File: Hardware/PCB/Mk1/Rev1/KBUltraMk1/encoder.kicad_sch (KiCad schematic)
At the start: 1 part, among them SW101 RotaryEncoder_Switch

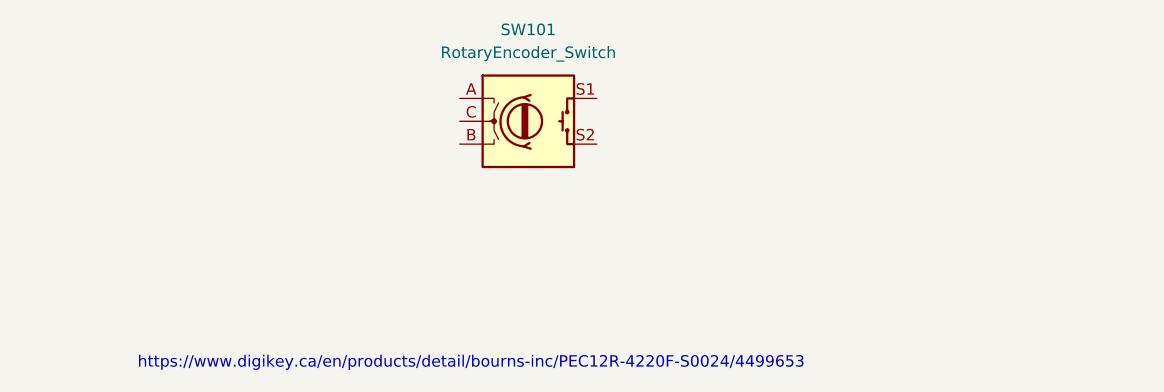
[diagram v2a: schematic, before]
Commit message: A
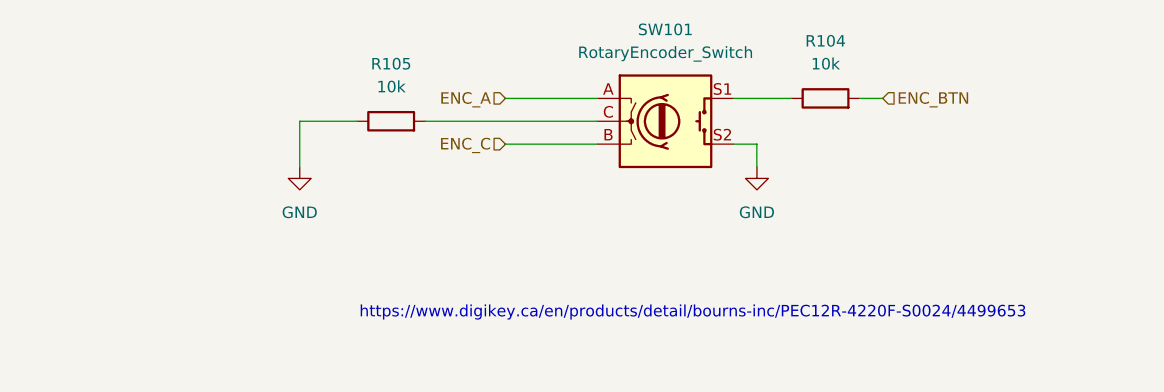
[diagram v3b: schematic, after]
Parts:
- added R104, R105: 10k, Resistor_SMD:R_0603_1608Metric, symbol Device:R
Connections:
- net ENC_A: now reaches SW101.A
- net ENC_C: now reaches SW101.B
- net at SW101.C: now also R105.2
- net at SW101.S1: now also R104.1
- net GND: now reaches SW101.S2
- net GND: now also R105.1
- new net ENC_BTN: R104.2
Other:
- moved on the sheet: SW101
